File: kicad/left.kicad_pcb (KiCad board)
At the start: 2 copper layers, 132 x 103 mm, 45 parts

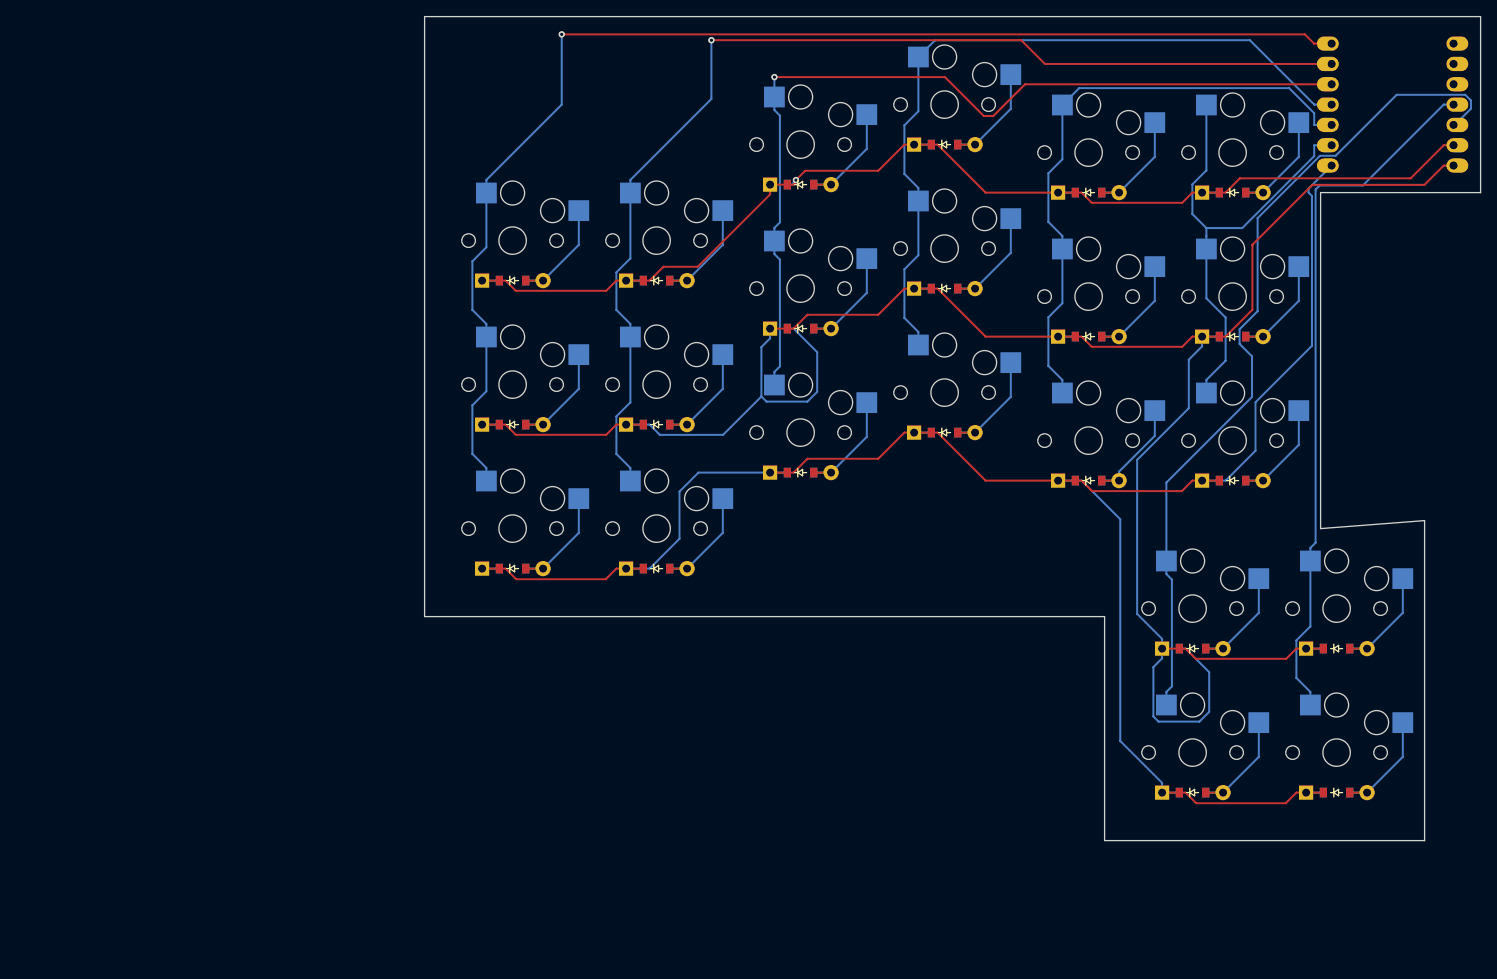
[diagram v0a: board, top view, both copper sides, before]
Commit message: reroute and do some other stuff I honestly forgot
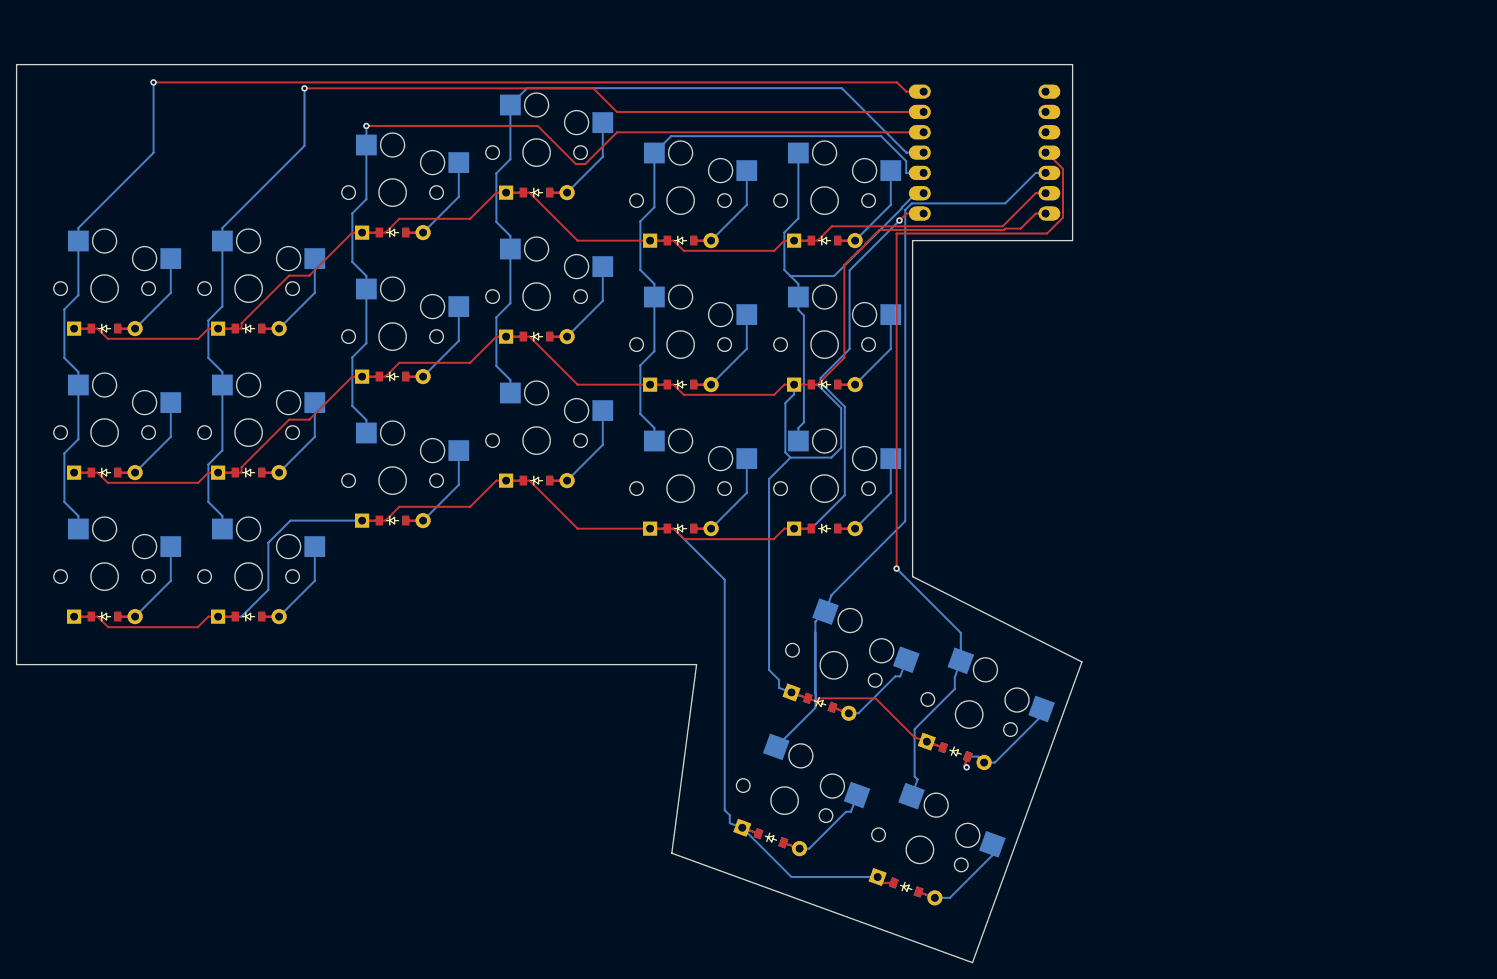
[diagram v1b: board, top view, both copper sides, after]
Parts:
- moved D21 55.1 mm to (232.2, 161.9), turned to -20 degrees
- moved S21 53.5 mm to (233.9, 157.2), turned to -20 degrees
- moved D19 53.0 mm to (215.3, 155.7), turned to -20 degrees
- moved D1 51.4 mm to (132.0, 128.0)
- moved D10 51.4 mm to (186.0, 111.0)
- moved D11 51.4 mm to (186.0, 93.0)
- moved D12 51.4 mm to (186.0, 75.0)
- moved D13 51.4 mm to (204.0, 117.0)
- moved D14 51.4 mm to (204.0, 99.0)
- moved D15 51.4 mm to (204.0, 81.0)
- moved D16 51.4 mm to (222.0, 117.0)
- moved D17 51.4 mm to (222.0, 99.0)
- moved D18 51.4 mm to (222.0, 81.0)
- moved D2 51.4 mm to (132.0, 110.0)
- moved D3 51.4 mm to (132.0, 92.0)
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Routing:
- net P7: track 274.2 -> 244.8 mm
- net P10: track 87.8 -> 106.9 mm, vias 0 -> 1
- net P6: track 235.8 -> 240.0 mm, vias 0 -> 1
- net P9: track 104.8 -> 101.8 mm
- net P2: track 112.9 -> 114.6 mm
- net P5: track 60.2 -> 59.0 mm
- net right_top: track 14.9 -> 15.9 mm, vias 0 -> 1
- net P8: track 148.7 -> 148.9 mm, vias 1 -> 0
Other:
- board size 132 x 103 mm -> 133.2 x 112.3 mm
